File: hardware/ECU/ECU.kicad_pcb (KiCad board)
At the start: 4 copper layers, 58 x 69 mm, 75 parts, among them IC1 IR4427SPBF, IC2 EL357NB_TA_-G, IC3 EL357NB_TA_-G, J1 USB_B_Micro, J2 TFP09-2-12B, J3 Connector, Q1 S8050, Q2 S8050, Q3 RJP63K2, Q4 RJP63K2, SW1 RESET, SW2 EN, U1 AMS1117-3.3, U2 AMS1117-3.3, U3 CP2102N-Axx-xQFN28, U4 ESP32-WROOM-32U

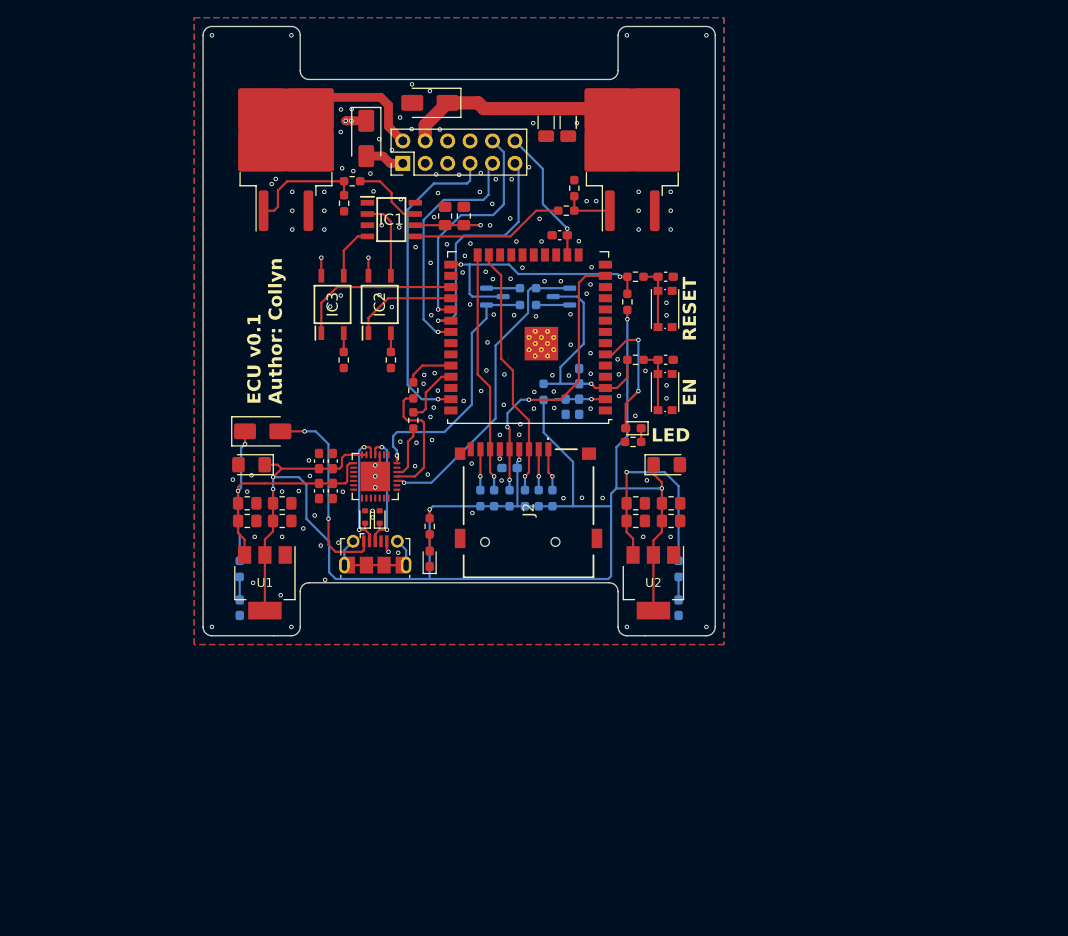
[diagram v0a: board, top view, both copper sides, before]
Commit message: ECU hardware v0.2 candidate
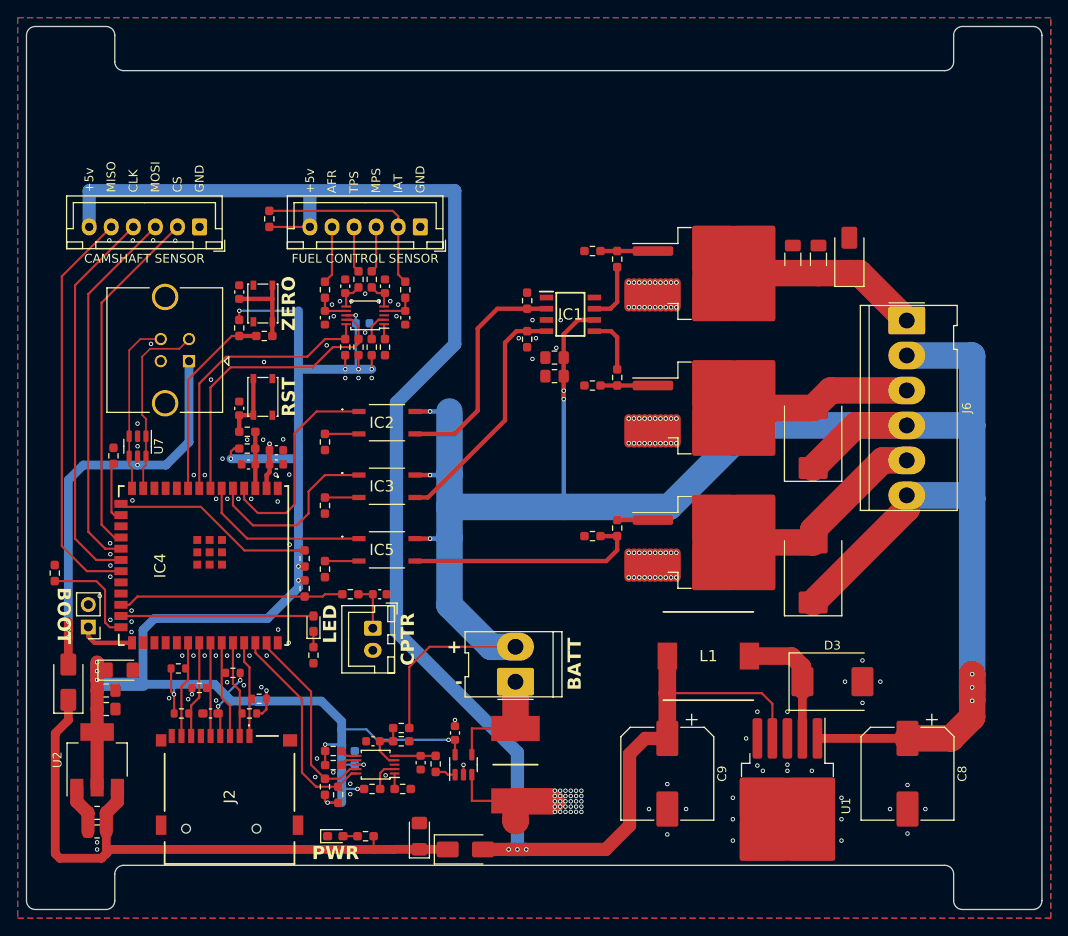
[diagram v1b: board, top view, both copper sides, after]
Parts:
- removed C15: 22u, Capacitor_SMD:C_0603_1608Metric_Pad1.08x0.95mm_HandSolder
- removed C22, C23: 1n, Capacitor_SMD:C_0603_1608Metric_Pad1.08x0.95mm_HandSolder
- removed D11: LED, LED_SMD:LED_0603_1608Metric_Pad1.05x0.95mm_HandSolder
- removed Q2: S8050, Package_TO_SOT_SMD:SOT-23
- removed U3: CP2102N-Axx-xQFN28, Package_DFN_QFN:QFN-28-1EP_5x5mm_P0.5mm_EP3.35x3.35mm
- added C24: 100n, Capacitor_SMD:C_0603_1608Metric, F.Cu at (154.6, 133.4)
- added C25: 100n, Capacitor_SMD:C_0603_1608Metric, F.Cu at (149.2, 130.9)
- added C26: 100n, Capacitor_SMD:C_0603_1608Metric, F.Cu at (150.0, 114.3)
- added C27: 100n, Capacitor_SMD:C_0603_1608Metric, F.Cu at (146.1, 79.4)
- added C28: 100n, Capacitor_SMD:C_0603_1608Metric, F.Cu at (150.6, 79.4)
- added C29: 100n, Capacitor_SMD:C_0603_1608Metric, F.Cu at (152.9, 83.0)
- added IC4: ESP32-S3-WROOM-1U-N8R8, MyLibrary:ESP32S3WROOM1UN4, F.Cu at (130.1, 111.0)
- added IC5: EL357NB_TA_-G, MyLibrary:EL357NG, F.Cu at (150.8, 109.3)
- added J4: USB_B, Connector_USB:USB_B_TE_5787834_Vertical, F.Cu at (128.4, 87.9)
- added J5: BATTERY, Connector_Molex:Molex_KK-396_5273-02A_1x02_P3.96mm_Vertical, F.Cu at (165.4, 124.2)
- added J6: GATEs, Connector_Molex:Molex_KK-396_5273-06A_1x06_P3.96mm_Vertical, F.Cu at (209.7, 83.3)
- added J8: CAPTURE_TRG, Connector_JST:JST_XH_B2B-XH-A_1x02_P2.50mm_Vertical, F.Cu at (149.2, 118.2)
- added JP1: BOOT, Connector_PinHeader_2.54mm:PinHeader_1x02_P2.54mm_Vertical, F.Cu at (117.0, 118.0)
- added L1: 100u, MyLibrary:INDPM102100X400N, F.Cu at (187.2, 121.3)
- added R26: 10k, Resistor_SMD:R_0603_1608Metric_Pad0.98x0.95mm_HandSolder, F.Cu at (146.1, 86.3)
- added R27: 100, Resistor_SMD:R_0603_1608Metric_Pad0.98x0.95mm_HandSolder, F.Cu at (135.0, 95.9)
- added R28: 100, Resistor_SMD:R_0603_1608Metric_Pad0.98x0.95mm_HandSolder, F.Cu at (136.9, 85.0)
- added R30: 1k, Resistor_SMD:R_0603_1608Metric_Pad0.98x0.95mm_HandSolder, F.Cu at (134.1, 84.1)
- added R31: 1k, Resistor_SMD:R_0603_1608Metric_Pad0.98x0.95mm_HandSolder, F.Cu at (142.5, 121.2)
- added R32: 10k, Resistor_SMD:R_0603_1608Metric_Pad0.98x0.95mm_HandSolder, F.Cu at (149.1, 86.3)
- added R33: 100, Resistor_SMD:R_0603_1608Metric_Pad0.98x0.95mm_HandSolder, F.Cu at (143.8, 79.8)
- added R34: 100, Resistor_SMD:R_0603_1608Metric_Pad0.98x0.95mm_HandSolder, F.Cu at (152.9, 79.8)
- added R35: 10k, Resistor_SMD:R_0603_1608Metric_Pad0.98x0.95mm_HandSolder, F.Cu at (150.6, 86.3)
- added R36: 100, Resistor_SMD:R_0603_1608Metric_Pad0.98x0.95mm_HandSolder, F.Cu at (149.1, 78.6)
- added R37: 100, Resistor_SMD:R_0603_1608Metric_Pad0.98x0.95mm_HandSolder, F.Cu at (147.6, 78.6)
- added R38: 0, Resistor_SMD:R_0603_1608Metric_Pad0.98x0.95mm_HandSolder, F.Cu at (176.9, 106.8)
- added R39: 100, Resistor_SMD:R_0603_1608Metric_Pad0.98x0.95mm_HandSolder, F.Cu at (156.3, 133.5)
- added R42: 10k, Resistor_SMD:R_0603_1608Metric_Pad0.98x0.95mm_HandSolder, F.Cu at (152.6, 136.3)
- added R43: 10k, Resistor_SMD:R_0603_1608Metric_Pad0.98x0.95mm_HandSolder, F.Cu at (149.1, 136.3)
- added R45: 0.01, MyLibrary:RESC10052X106N, F.Cu at (165.4, 133.6)
- added R47: 130k, Resistor_SMD:R_0603_1608Metric_Pad0.98x0.95mm_HandSolder, F.Cu at (152.4, 129.4)
- added R50: 5.6k, Resistor_SMD:R_0603_1608Metric_Pad0.98x0.95mm_HandSolder, F.Cu at (152.4, 130.9)
- added R51: 10k, Resistor_SMD:R_0603_1608Metric_Pad0.98x0.95mm_HandSolder, F.Cu at (144.7, 133.7)
- added R52: 1k, Resistor_SMD:R_0603_1608Metric_Pad0.98x0.95mm_HandSolder, F.Cu at (146.7, 114.3)
- added R53: 1k, Resistor_SMD:R_0603_1608Metric_Pad0.98x0.95mm_HandSolder, F.Cu at (141.5, 113.7)
- added R54: 1k, Resistor_SMD:R_0603_1608Metric_Pad0.98x0.95mm_HandSolder, F.Cu at (137.5, 71.8)
- added U5: ADS1115IDGS, Package_SO:TSSOP-10_3x3mm_P0.5mm, F.Cu at (149.5, 133.6)
- added U6: INA180A3, Package_TO_SOT_SMD:SOT-23-5, F.Cu at (159.5, 133.6)
- added U7: SRV05-4, Package_TO_SOT_SMD:SOT-23-6, F.Cu at (122.6, 97.5)
- C10, C12: value 10u -> 100n; footprint Capacitor_SMD:C_0603_1608Metric_Pad1.08x0.95mm_HandSolder -> Capacitor_SMD:C_0603_1608Metric
- C11: footprint Capacitor_SMD:C_0603_1608Metric_Pad1.08x0.95mm_HandSolder -> Capacitor_SMD:C_0603_1608Metric
- C13: value 1n -> 100n; footprint Capacitor_SMD:C_0603_1608Metric_Pad1.08x0.95mm_HandSolder -> Capacitor_SMD:C_0603_1608Metric
- C14: footprint Capacitor_SMD:C_0603_1608Metric_Pad1.08x0.95mm_HandSolder -> Capacitor_SMD:C_0603_1608Metric; moved to F.Cu
- C16, D1, R2: moved to F.Cu
- C21: value 1n -> 100n; footprint Capacitor_SMD:C_0603_1608Metric_Pad1.08x0.95mm_HandSolder -> Capacitor_SMD:C_0603_1608Metric; moved to B.Cu
- C3, C4: footprint Capacitor_SMD:C_0805_2012Metric_Pad1.18x1.45mm_HandSolder -> Capacitor_SMD:C_0603_1608Metric
- C5: value 100n -> 1u; footprint Capacitor_SMD:C_0805_2012Metric_Pad1.18x1.45mm_HandSolder -> Capacitor_SMD:C_0603_1608Metric
- C8: value 22u -> 100u; footprint Capacitor_SMD:C_0805_2012Metric_Pad1.18x1.45mm_HandSolder -> Capacitor_SMD:CP_Elec_10x10
- C9: value 100n -> 1n; footprint Capacitor_SMD:C_0603_1608Metric_Pad1.08x0.95mm_HandSolder -> Capacitor_SMD:CP_Elec_10x10
- D10: value 1n4007 -> m7
- D3: value LED -> ss36; footprint LED_SMD:LED_0603_1608Metric_Pad1.05x0.95mm_HandSolder -> Diode_SMD:D_SMC; moved to F.Cu
- D4: value 3.6v -> 5v
- D5: value 1n4001 -> LED; footprint Diode_SMD:D_SMA -> LED_SMD:LED_0603_1608Metric_Pad1.05x0.95mm_HandSolder
- D6: value 5v -> ss36; footprint Diode_SMD:D_SOD-523 -> Diode_SMD:D_SMC
- D7: value 5v -> m7; footprint Diode_SMD:D_SOD-523 -> Diode_SMD:D_SMA
- D8: value LED -> ss36; footprint LED_SMD:LED_0603_1608Metric_Pad1.05x0.95mm_HandSolder -> Diode_SMD:D_SMC
- IC1: footprint My_Lirbrary:SOIC127P600X175-8N -> MyLibrary:SOIC127P600X175-8N
- IC2, IC3: footprint My_Lirbrary:SOP254P700X200-4N -> MyLibrary:EL357NG
- J1: value USB_B_Micro -> AQS; footprint Connector_USB:USB_Micro-B_Molex-105017-0001 -> Connector_JST:JST_XH_B6B-XH-A_1x06_P2.50mm_Vertical
- J2: footprint My_Lirbrary:TFP09212B -> MyLibrary:TFP09212B
- J3: value Connector -> CAM_SENSOR; footprint Connector_PinHeader_2.54mm:PinHeader_2x06_P2.54mm_Vertical -> Connector_JST:JST_XH_B6B-XH-A_1x06_P2.50mm_Vertical
- Q1: value S8050 -> RJP63K2; footprint Package_TO_SOT_SMD:SOT-23 -> Package_TO_SOT_SMD:TO-263-2; moved to F.Cu
- R1: value 1M -> 10k; moved to F.Cu
- R16, R17, R18, R19, R20, R21: footprint Resistor_SMD:R_0603_1608Metric_Pad0.98x0.95mm_HandSolder -> Resistor_SMD:R_0603_1608Metric; moved to F.Cu
- R22, R23: value 470 -> 10k
- R24: value 5k -> 10k
- R25: value 1k -> 10k
- R3: value 2k -> 10k; moved to F.Cu
- R4, R5, R8: value 12k -> 10k; moved to F.Cu
- R6, R7: value 0 -> 10k
- R9: value 2k -> 100
- SW1: value RESET -> RESET BTN; footprint Button_Switch_SMD:SW_Push_1P1T_NO_CK_KMR2 -> Button_Switch_SMD:SW_SPST_PTS810
- SW2: value EN -> ZERO BTN; footprint Button_Switch_SMD:SW_Push_1P1T_NO_CK_KMR2 -> Button_Switch_SMD:SW_SPST_PTS810
- U1: value AMS1117-3.3 -> LM2576S-5; footprint Package_TO_SOT_SMD:SOT-223-3_TabPin2 -> Package_TO_SOT_SMD:TO-263-5_TabPin3
- U4: value ESP32-WROOM-32U -> ADS1115IDGS; footprint RF_Module:ESP32-WROOM-32U -> Package_SO:TSSOP-10_3x3mm_P0.5mm
- moved D10 81.3 mm to (159.7, 143.2), turned to 0 degrees
- moved C8 77.2 mm to (209.8, 134.6), turned to -90 degrees
- moved C2 70.4 mm to (118.0, 141.2), turned to 180 degrees
- moved C7 70.4 mm to (118.0, 139.1), turned to 180 degrees
- moved D3 67.6 mm to (201.3, 124.2), turned to 0 degrees
- moved C6 67.4 mm to (119.0, 127.3)
- moved C1 67.4 mm to (119.0, 125.2)
- moved U2 66.1 mm to (118.0, 133.1), turned to 90 degrees
- moved U1 64.3 mm to (196.2, 138.3)
- moved R22 62.5 mm to (119.8, 98.6), turned to 90 degrees
- moved R5 61.0 mm to (143.8, 136.1), turned to 90 degrees
- moved R24 60.8 mm to (144.7, 132.1), turned to 180 degrees
- moved R4 59.5 mm to (145.3, 137.0), turned to 90 degrees
- moved R8 59.0 mm to (113.2, 111.9)
- moved Q4 57.6 mm to (188.6, 93.2), turned to 0 degrees
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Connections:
- net Net-(J2-CD/DAT3) renamed /SD_DAT3
- net Net-(J2-DAT2) renamed /SD_DAT2
- C10 pad 1: VBUS -> GND
- C10 pad 2: GND -> +3.3V
- C11 pad 1: +3.3V -> GND
- C11 pad 2: GND -> Net-(C11-Pad2)
- C12 pad 1: +3.3V -> GND
- C12 pad 2: GND -> Net-(C12-Pad2)
- C13 pad 1: /EN -> GND
- C13 pad 2: GND -> +3.3V
- C14 pad 2: +3.3V -> Net-(U4-AIN3)
- C18 pad 1: +12V -> +BATT
- C19 pad 1: +12V -> +BATT
- C2 pad 1: +12V -> +4V
- C21 pad 2: /O2 -> +3.3V
- C3 pad 1: VBUS -> GND
- C3 pad 2: GND -> +3.3V
- C4 pad 1: VBUS -> GND
- C4 pad 2: GND -> +3.3V
- C5 pad 1: +3.3V -> GND
- C5 pad 2: GND -> /RESET_PIN
- C7 pad 1: +12V -> +4V
- C8 pad 1: +3.3V -> +BATT
- C9 pad 1: VBUS -> +5V
- D10 pad 1: +12V -> +4V
- D10 pad 2: +BATT -> +5V
- D3 pad 1: GND -> Net-(D3-K)
- D3 pad 2: Net-(D3-A) -> GND
- D4 pad 1: +3.3V -> +4V
- D5 pad 1: VBUS -> Net-(D5-K)
- D5 pad 2: Net-(D5-A) -> /LED_PIN
- D6 pad 1: Net-(D6-K) -> +BATT
- D6 pad 2: GND -> /FUEL
- D7 pad 1: Net-(D7-K) -> +4V
- D7 pad 2: GND -> Net-(D7-A)
- D8 pad 1: GND -> +BATT
- D8 pad 2: Net-(D8-A) -> /PUMP
- IC1 pad 5: /COIL_IGBT -> Net-(IC1-OUT_B)
- IC1 pad 6: +12V -> +BATT
- IC1 pad 7: /FUEL_IGBT -> Net-(IC1-OUT_A)
- IC2 pad 1: /FUEL_PIN -> /COIL_PIN
- IC2 pad 4: +12V -> +BATT
- IC3 pad 1: /COIL_PIN -> /FUEL_PIN
- IC3 pad 4: +12V -> +BATT
- J1 pad 1: Net-(D5-A) -> GND
- J1 pad 2: Net-(D6-K) -> /IAT
- J1 pad 3: Net-(D7-K) -> /MPS
- J1 pad 4: unconnected-(J1-ID-Pad4) -> /TPS
- J1 pad 5: GND -> /AFR
- J1 pad 6: Net-(J1-Shield) -> +5V
- J2 pad 8: Net-(J2-DAT1) -> /SD_DAT1
- J3 pad 1: +BATT -> GND
- J3 pad 2: /FUEL -> /FSPI_CS
- J3 pad 3: GND -> /FSPI_MOSI
- J3 pad 4: /COIL -> /FSPI_CLK
- J3 pad 5: GND -> /FSPI_MISO
- J3 pad 6: GND -> +5V
- Q1 pad 1: Net-(Q1-E) -> Net-(Q1-G)
- Q1 pad 2: Net-(Q1-B) -> /PUMP
- Q1 pad 3: /EN -> GND
- R1 pad 1: Net-(J1-Shield) -> GND
- R1 pad 2: GND -> Net-(IC1-INA)
- R11 pad 2: /COIL_IGBT -> Net-(IC1-OUT_A)
- R15 pad 2: /FUEL_IGBT -> Net-(IC1-OUT_B)
- R2 pad 1: +12V -> +4V
- R21 pad 1: Net-(J2-DAT1) -> +3.3V
- R21 pad 2: +3.3V -> /SD_DAT1
- R22 pad 1: Net-(C22-Pad1) -> Net-(IC4-IO46)
- R22 pad 2: /IO0 -> GND
- R23 pad 1: Net-(C23-Pad1) -> GND
- R23 pad 2: /EN -> Net-(IC5-E)
- R24 pad 1: /IO0 -> Net-(U5-AIN2)
- R25 pad 1: GND -> /SDA_0
- R25 pad 2: Net-(D11-K) -> +3.3V
- R3 pad 1: VBUS -> GND
- R3 pad 2: Net-(D3-A) -> Net-(IC1-INB)
- R4 pad 1: Net-(Q2-E) -> +3.3V
- R4 pad 2: Net-(Q1-B) -> /SCL_1
- R5 pad 1: Net-(Q1-E) -> +3.3V
- R5 pad 2: Net-(Q2-B) -> /SDA_1
- R6 pad 1: Net-(U3-RXD) -> /RESET_PIN
- R6 pad 2: /RXD -> +3.3V
- R7 pad 2: /TXD -> +3.3V
- R8 pad 1: /EN -> GND
- R8 pad 2: +3.3V -> Net-(IC4-IO45)
- R9 pad 1: +3.3V -> GND
- R9 pad 2: Net-(D8-A) -> Net-(IC5-K)
- SW1 pad 2: Net-(C22-Pad1) -> Net-(C11-Pad2)
- SW2 pad 2: Net-(C23-Pad1) -> Net-(C12-Pad2)
- U1 pad 1: GND -> +BATT
- U1 pad 2: +3.3V -> Net-(D3-K)
- U1 pad 3: VBUS -> GND
- U2 pad 3: +12V -> +4V
- U4 pad 1: GND -> Net-(U4-ADDR)
- U4 pad 10: unconnected-(U4-IO25-Pad10) -> /SCL_0
- U4 pad 2: +3.3V -> Net-(U4-ALERT/RDY)
- U4 pad 3: /EN -> GND
- U4 pad 4: unconnected-(U4-SENSOR_VP-Pad4) -> Net-(U4-AIN0)
- U4 pad 5: unconnected-(U4-SENSOR_VN-Pad5) -> Net-(U4-AIN1)
- U4 pad 7: unconnected-(U4-IO35-Pad7) -> Net-(U4-AIN3)
- U4 pad 8: unconnected-(U4-IO32-Pad8) -> +3.3V
- U4 pad 9: unconnected-(U4-IO33-Pad9) -> /SDA_0
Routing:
- net +BATT: track 4.48 -> 257.3 mm, vias 0 -> 8
- net +5V: track 0.00 -> 195.7 mm, vias 0 -> 3
- net GND: track 3.96 -> 105.0 mm, vias 157 -> 195
- net +4V: track 0.00 -> 72.6 mm
- net Net-(D7-A): track 0.00 -> 48.3 mm, vias 0 -> 4
- net /FSPI_MISO: track 0.00 -> 46.3 mm
- net /FSPI_CLK: track 0.00 -> 44.2 mm
- net /FSPI_MOSI: track 0.00 -> 42.2 mm
- net /FSPI_CS: track 0.00 -> 40.1 mm
- net +12V: track 38.6 -> 0.00 mm, vias 6 -> 0
- net VBUS: track 38.3 -> 0.00 mm, vias 2 -> 0
- net /VSPI_MOSI: track 35.8 -> 0.00 mm, vias 1 -> 0
- net Net-(Q1-E): track 35.1 -> 0.00 mm, vias 1 -> 0
- net /SDA_0: track 0.00 -> 33.9 mm
- net /SCL_0: track 0.00 -> 32.2 mm
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- removed copper zone on In2.Cu, net +12V
- removed copper zone on In1.Cu, net GND
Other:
- board size 58 x 69 mm -> 115 x 100 mm
- copper layers 4 -> 2
- board text added: "+"
- board text added: "+5v"
- board text added: "-"
- board text added: "AFR"
- board text added: "BOOT"
- board text added: "CAMSHAFT SENSOR"
- board text added: "CPTR"
- board text added: "ECU v0.2 Author: Collyn"
- board text added: "FUEL CONTROL SENSOR"
- board text added: "IAT"
- board text added: "MPS"
- board text added: "PWR"
- board text added: "RST"
- board text added: "TPS"
- board text added: "ZERO"
- board text removed: "COIL"
- board text removed: "ECU v0.1 Author: Collyn"
- board text removed: "EN"
- board text removed: "FUEL"
- board text removed: "O2"
- board text removed: "RESET"
